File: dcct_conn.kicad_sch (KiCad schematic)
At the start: 1 part, among them J6 1731130154

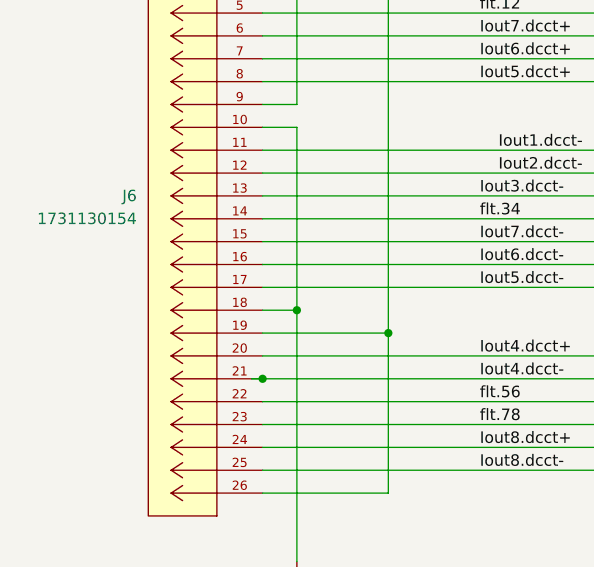
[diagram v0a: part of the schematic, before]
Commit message: Start routing
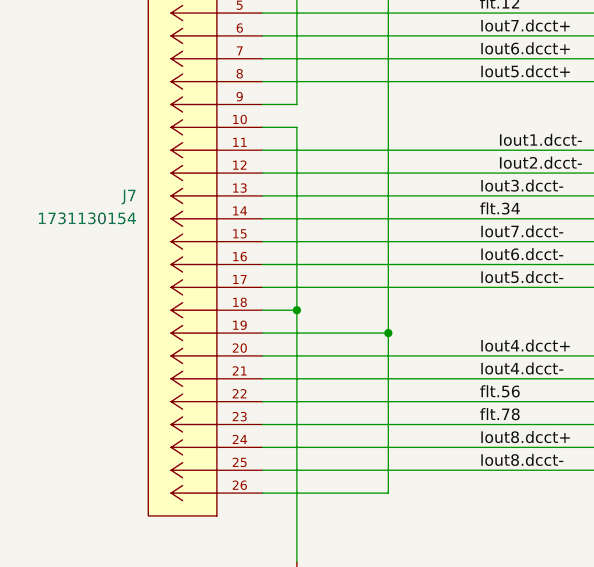
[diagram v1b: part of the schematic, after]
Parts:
- renumbered J6 to J7
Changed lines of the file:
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@@
-	)
-	(junction
-		(at 90.17 125.73)
-		(diameter 0)
-		(color 0 0 0 0)
 	)
 	(junction
@@
 	(wire
 		(pts
-			(xy 88.9 125.73) (xy 90.17 125.73)
-		)
-		(stroke
-			(width 0)
-			(type default)
-		)
-	)
-	(wire
-		(pts
 			(xy 90.17 77.47) (xy 142.24 77.47)
 		)
@@
 	(wire
 		(pts
+			(xy 90.17 85.09) (xy 167.64 85.09)
+		)
+		(stroke
+			(width 0)
+			(type default)
+		)
+	)
+	(wire
+		(pts
 			(xy 104.14 71.12) (xy 104.14 120.65)
 		)
@@
 	(wire
 		(pts
+			(xy 90.17 125.73) (xy 153.67 125.73)
+		)
+		(stroke
+			(width 0)
+			(type default)
+		)
+	)
+	(wire
+		(pts
 			(xy 90.17 107.95) (xy 167.64 107.95)
 		)
@@
 	(wire
 		(pts
-			(xy 90.17 125.73) (xy 153.67 125.73)
+			(xy 167.64 85.09) (xy 175.26 85.09)
 		)
 		(stroke
@@
 	(wire
 		(pts
-			(xy 90.17 85.09) (xy 167.64 85.09)
-		)
-		(stroke
-			(width 0)
-			(type default)
-		)
-	)
-	(wire
-		(pts
 			(xy 104.14 120.65) (xy 90.17 120.65)
 		)
@@
 		(pts
 			(xy 171.45 130.81) (xy 175.26 130.81)
-		)
-		(stroke
-			(width 0)
-			(type default)
-		)
-	)
-	(wire
-		(pts
-			(xy 167.64 85.09) (xy 175.26 85.09)
 		)
 		(stroke
@@
 		(on_board yes)
 		(dnp no)
-		(property "Reference" "J6"
+		(property "Reference" "J7"
 			(at 76.2 105.4099 0)
 			(effects
@@
 			(project "psc_carrier_brd"
 				(path "/40891cc8-bf64-41f4-8f69-a607d7b280eb/ee7775f8-818d-4b39-ac35-648c0c49495f"
-					(reference "J6")
+					(reference "J7")
 					(unit 1)
 				)
@@
 		(dnp no)
 		(fields_autoplaced yes)
-		(property "Reference" "#PWR030"
+		(property "Reference" "#PWR031"
 			(at 93.98 152.4 0)
 			(effects
@@
 			(project ""
 				(path "/40891cc8-bf64-41f4-8f69-a607d7b280eb/ee7775f8-818d-4b39-ac35-648c0c49495f"
-					(reference "#PWR030")
+					(reference "#PWR031")
 					(unit 1)
 				)
@@
 		(dnp no)
 		(fields_autoplaced yes)
-		(property "Reference" "#PWR031"
+		(property "Reference" "#PWR032"
 			(at 104.14 74.93 0)
 			(effects
@@
 			(project ""
 				(path "/40891cc8-bf64-41f4-8f69-a607d7b280eb/ee7775f8-818d-4b39-ac35-648c0c49495f"
-					(reference "#PWR031")
+					(reference "#PWR032")
 					(unit 1)
 				)
@@
 		(dnp no)
 		(fields_autoplaced yes)
-		(property "Reference" "#PWR029"
+		(property "Reference" "#PWR030"
 			(at 93.98 72.39 0)
 			(effects
@@
 			(project ""
 				(path "/40891cc8-bf64-41f4-8f69-a607d7b280eb/ee7775f8-818d-4b39-ac35-648c0c49495f"
-					(reference "#PWR029")
+					(reference "#PWR030")
 					(unit 1)
 				)

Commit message: Finished layout
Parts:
- J7: Cost (none) -> 24.50; MFG (none) -> Molex; MFG_PN (none) -> 1731130154
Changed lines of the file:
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@@
 			)
 		)
-		(property "Description" ""
+		(property "Description" "CONN D-SUB HD PLG 26POS R/A SLDR"
 			(at 90.17 74.93 0)
 			(effects
@@
 				(hide yes)
 			)
+		)
+		(property "Cost" "24.50"
+			(at 90.17 74.93 0)
+			(effects
+				(font
+					(size 1.27 1.27)
+				)
+				(hide yes)
+			)
+		)
+		(property "MFG" "Molex"
+			(at 90.17 74.93 0)
+			(effects
+				(font
+					(size 1.27 1.27)
+				)
+				(hide yes)
+			)
+		)
+		(property "MFG_PN" "1731130154"
+			(at 90.17 74.93 0)
+			(effects
+				(font
+					(size 1.27 1.27)
+				)
+				(hide yes)
+			)
